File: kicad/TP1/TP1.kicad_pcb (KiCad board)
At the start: 2 copper layers, 21 parts, among them P1 CONN_20X2, P2 CONN_20X2, U1 MPU-6050, U2 CR2013-MI2120, U4 LM386

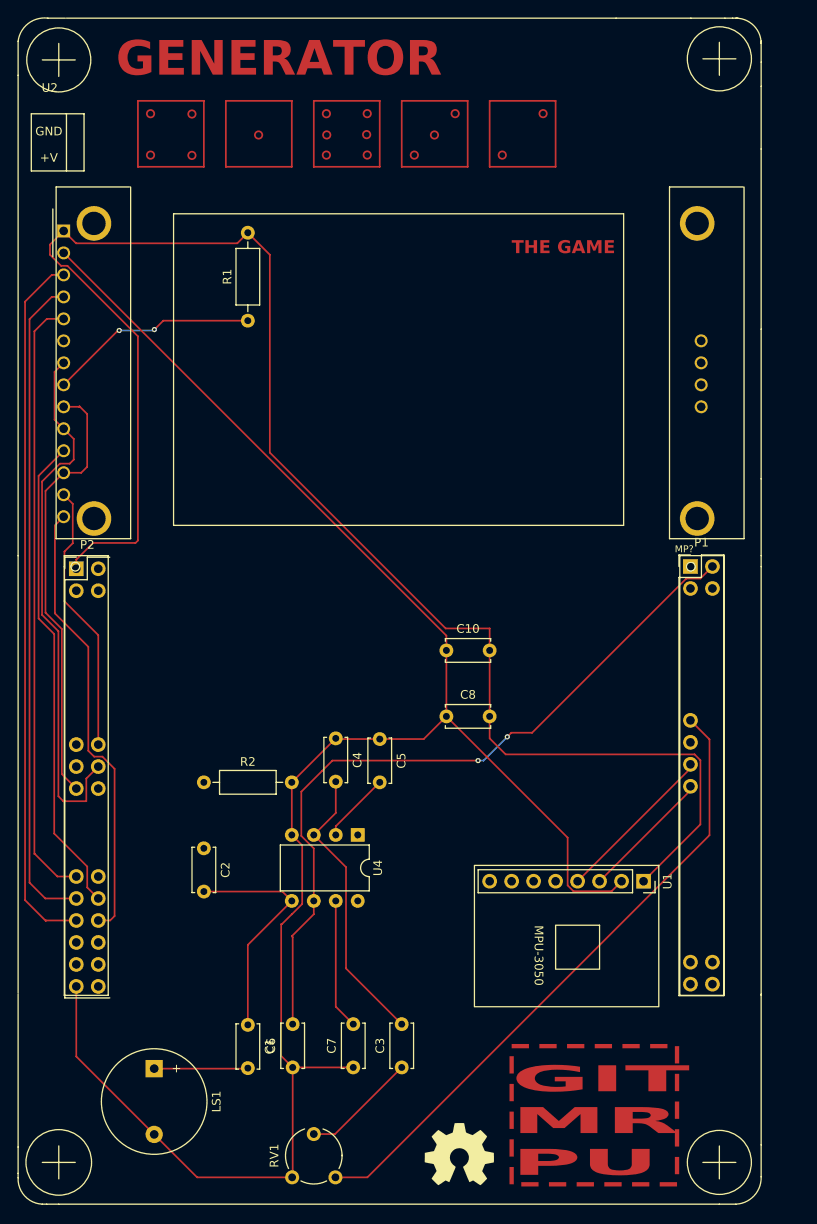
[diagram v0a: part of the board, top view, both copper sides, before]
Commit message: Actualizacion de KiCad
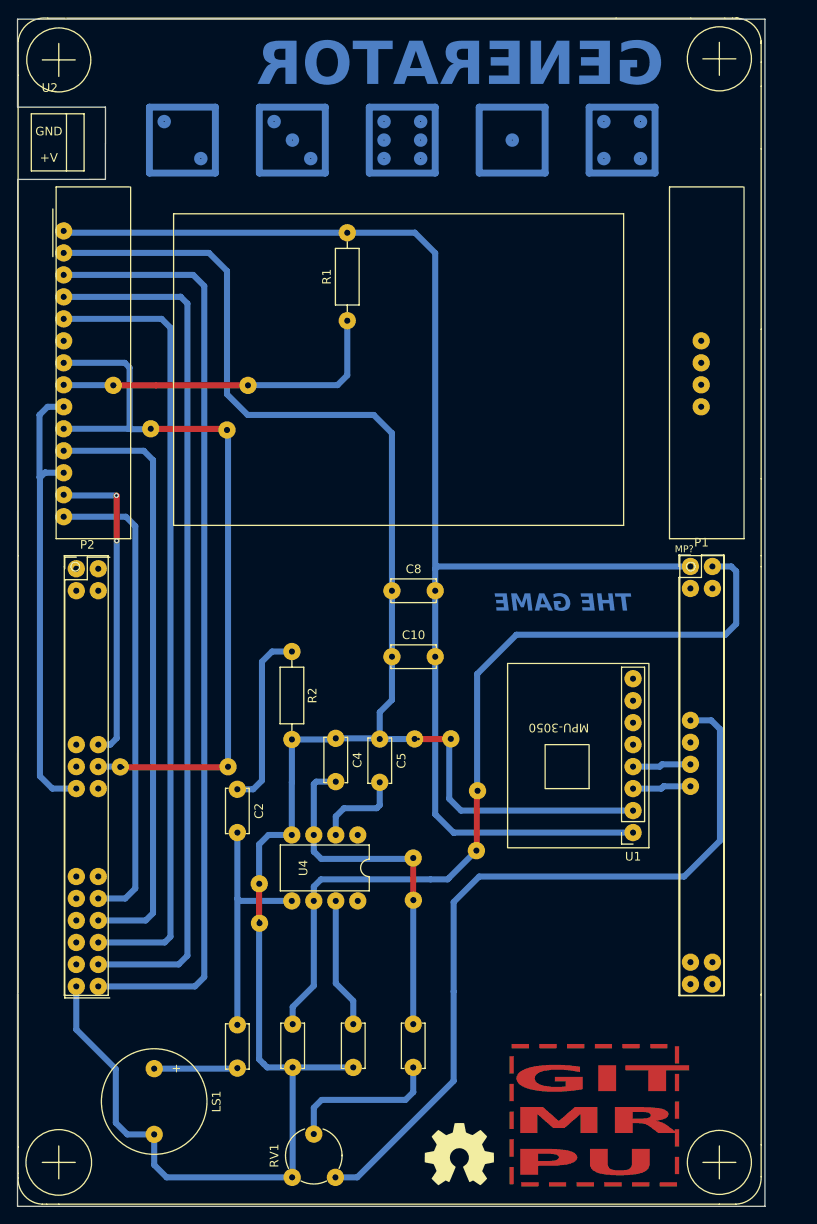
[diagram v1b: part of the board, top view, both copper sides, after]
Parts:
- added ?: , , F.Cu at (64.4, 75.3)
- added ?: , , F.Cu at (65.2, 119.4)
- added ?: , , F.Cu at (103.4, 116.2)
- added ?: , , F.Cu at (81.3, 132.9)
- added ?: , , F.Cu at (81.3, 137.5)
- added ?: , , F.Cu at (77.5, 80.5)
- added ?: , , F.Cu at (80.0, 75.3)
- added ?: , , F.Cu at (68.7, 80.3)
- added ?: , , F.Cu at (99.1, 134.8)
- added ?: , , F.Cu at (99.1, 129.9)
- added ?: , , F.Cu at (106.4, 129.1)
- added ?: , , F.Cu at (106.5, 122.2)
- added ?: , , F.Cu at (99.2, 116.2)
- added ?: , , F.Cu at (77.7, 119.4)
- moved R2 18.2 mm to (85.0, 106.1), turned to -90 degrees
- moved C8 15.8 mm to (96.6, 99.1)
- moved R1 11.5 mm to (91.4, 67.9)
- moved C2 7.84 mm to (78.7, 122.0)
- moved C10 6.33 mm to (96.6, 106.7)
- moved U1 5.75 mm to (124.5, 127.0), turned to 180 degrees
- moved C3 1.33 mm to (99.1, 154.1)
- moved C1 1.21 mm to (78.7, 149.2)
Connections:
- P1 pad 1: unconnected-(P1-P1-Pad1) -> +3.3V
- P2 pad 1: +3.3V -> unconnected-(P2-P1-Pad1)
- P2 pad 29: GPIO_0 -> unconnected-(P2-P29-Pad29)
- P2 pad 31: GPIO_2 -> unconnected-(P2-P31-Pad31)
- P2 pad 33: GPIO_4 -> unconnected-(P2-P33-Pad33)
- P2 pad 35: GPIO_6 -> unconnected-(P2-P35-Pad35)
- P2 pad 36: unconnected-(P2-P36-Pad36) -> GPIO_5
- P2 pad 38: unconnected-(P2-P38-Pad38) -> GPIO_7
- P2 pad 40: unconnected-(P2-P40-Pad40) -> GPIO_8
- U2 pad 11: GPIO_0 -> GPIO_5
- U2 pad 12: GPIO_2 -> GPIO_7
- U2 pad 13: GPIO_4 -> GPIO_8
- U2 pad 2: GPIO_3 -> GPIO_1
- U2 pad 5: GPIO_1 -> GPIO_3
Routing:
- net GPIO_8: track 0.00 -> 109.3 mm
- net GPIO_7: track 0.00 -> 100.7 mm
- net GPIO_5: track 0.00 -> 91.7 mm
- net GPIO_4: track 81.8 -> 0.00 mm
- net GPIO_2: track 76.3 -> 0.00 mm
- net GPIO_0: track 70.3 -> 0.00 mm
- net GND: track 218.9 -> 244.6 mm, vias 0 -> 4
- net SPI_SCK: track 62.4 -> 88.0 mm, vias 0 -> 4
- net +3.3V: track 187.6 -> 162.2 mm
- net Net-(C2-Pad1): track 0.00 -> 20.9 mm
- net GPIO_3: track 52.1 -> 69.8 mm
- net DAC: track 73.8 -> 89.4 mm
- net Net-(U2-LED): track 24.3 -> 39.6 mm
- net +5V: track 86.8 -> 99.3 mm
- net I2C_SDA: track 18.9 -> 6.75 mm
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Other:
- board outline added: 86.4 x 137.2 mm
